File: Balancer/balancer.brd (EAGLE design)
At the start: 170 x 230 mm, 285 parts, among them Q1 BSS123W, Q10A SIR882DP-T1-GE3, Q10B SIS468DN-T1-GE3, Q11A SIR882DP-T1-GE3, Q11B SIS468DN-T1-GE3, Q12A SIR882DP-T1-GE3, Q12B SIS468DN-T1-GE3, Q2 BSS123W, Q3A SIR882DP-T1-GE3, Q3B SIS468DN-T1-GE3, Q4 MMBT3906LT1G, Q4A SIR882DP-T1-GE3, Q4B SIS468DN-T1-GE3, Q5 FDN5618P, Q5A SIR882DP-T1-GE3, Q5B SIS468DN-T1-GE3, Q6 CMPT3904E_TR_PBFREE, Q6A SIR882DP-T1-GE3, Q6B SIS468DN-T1-GE3, Q9A SIR882DP-T1-GE3, Q9B SIS468DN-T1-GE3, T10 750312504, T11 750312504, T12 750312504, T3 750312504, T4 750312504, T5 750312504, T6 750312504, T9 750312504, U1 LTC3300ILXE-1PBF, U2 LTC3300ILXE-1PBF

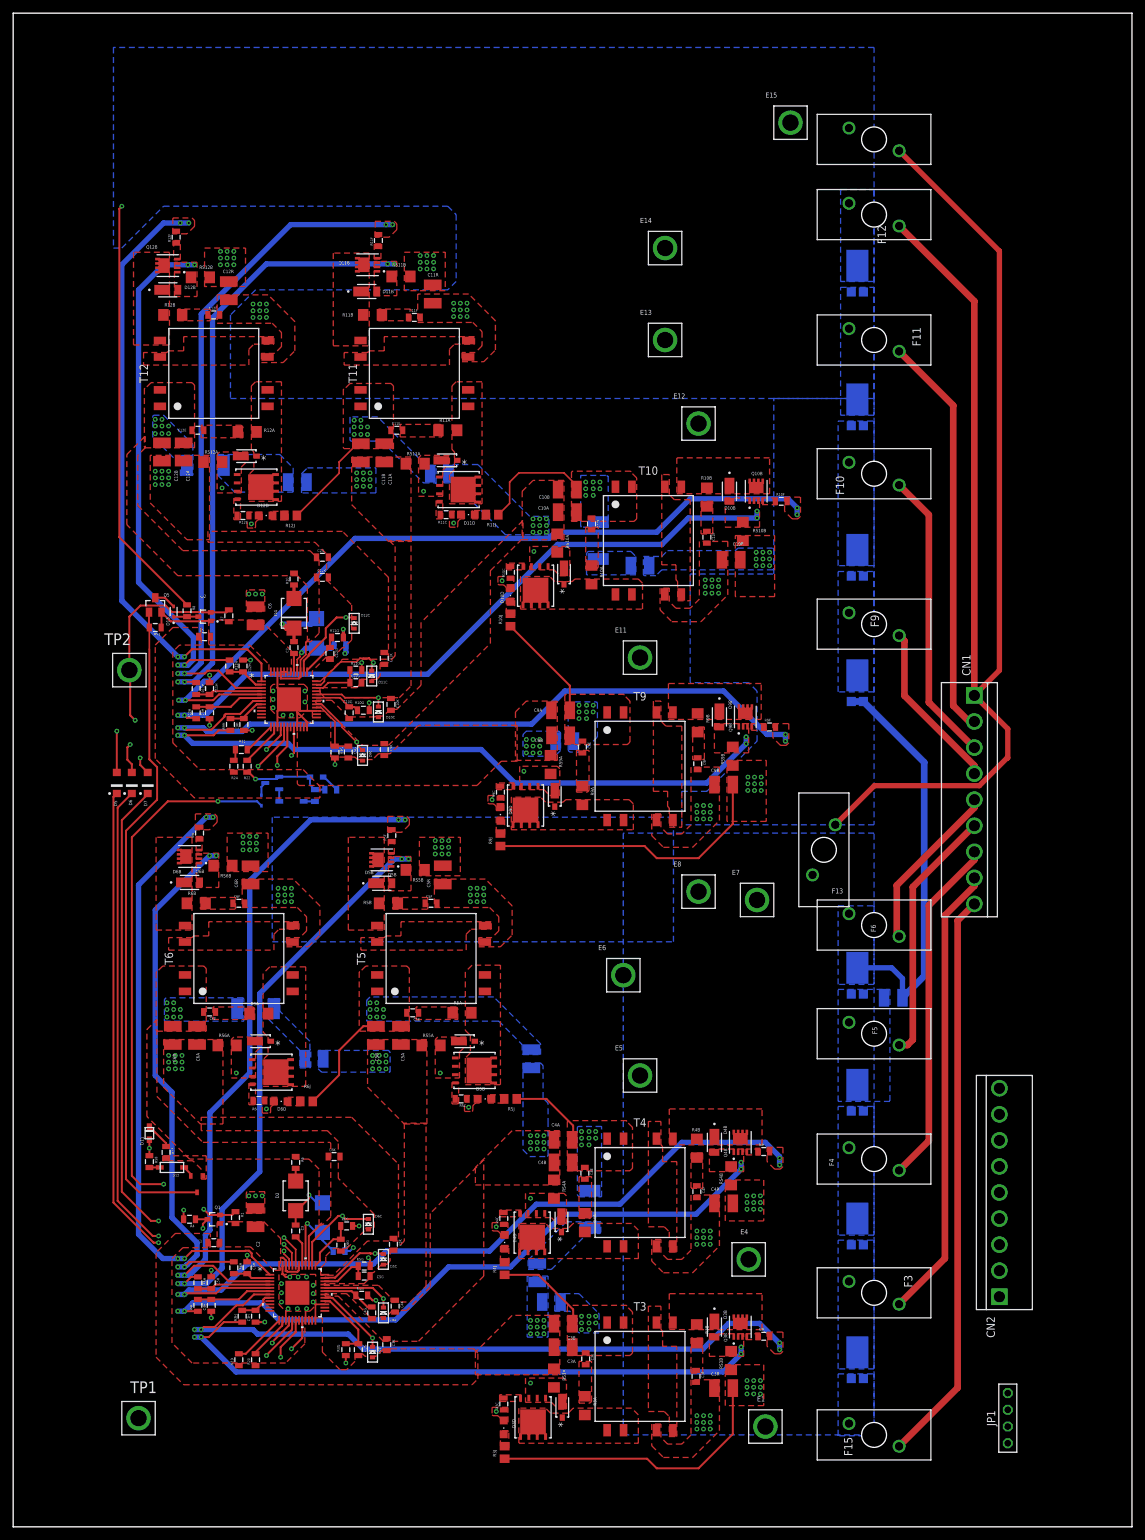
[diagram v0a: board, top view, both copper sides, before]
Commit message: done final check, generated Gerber file
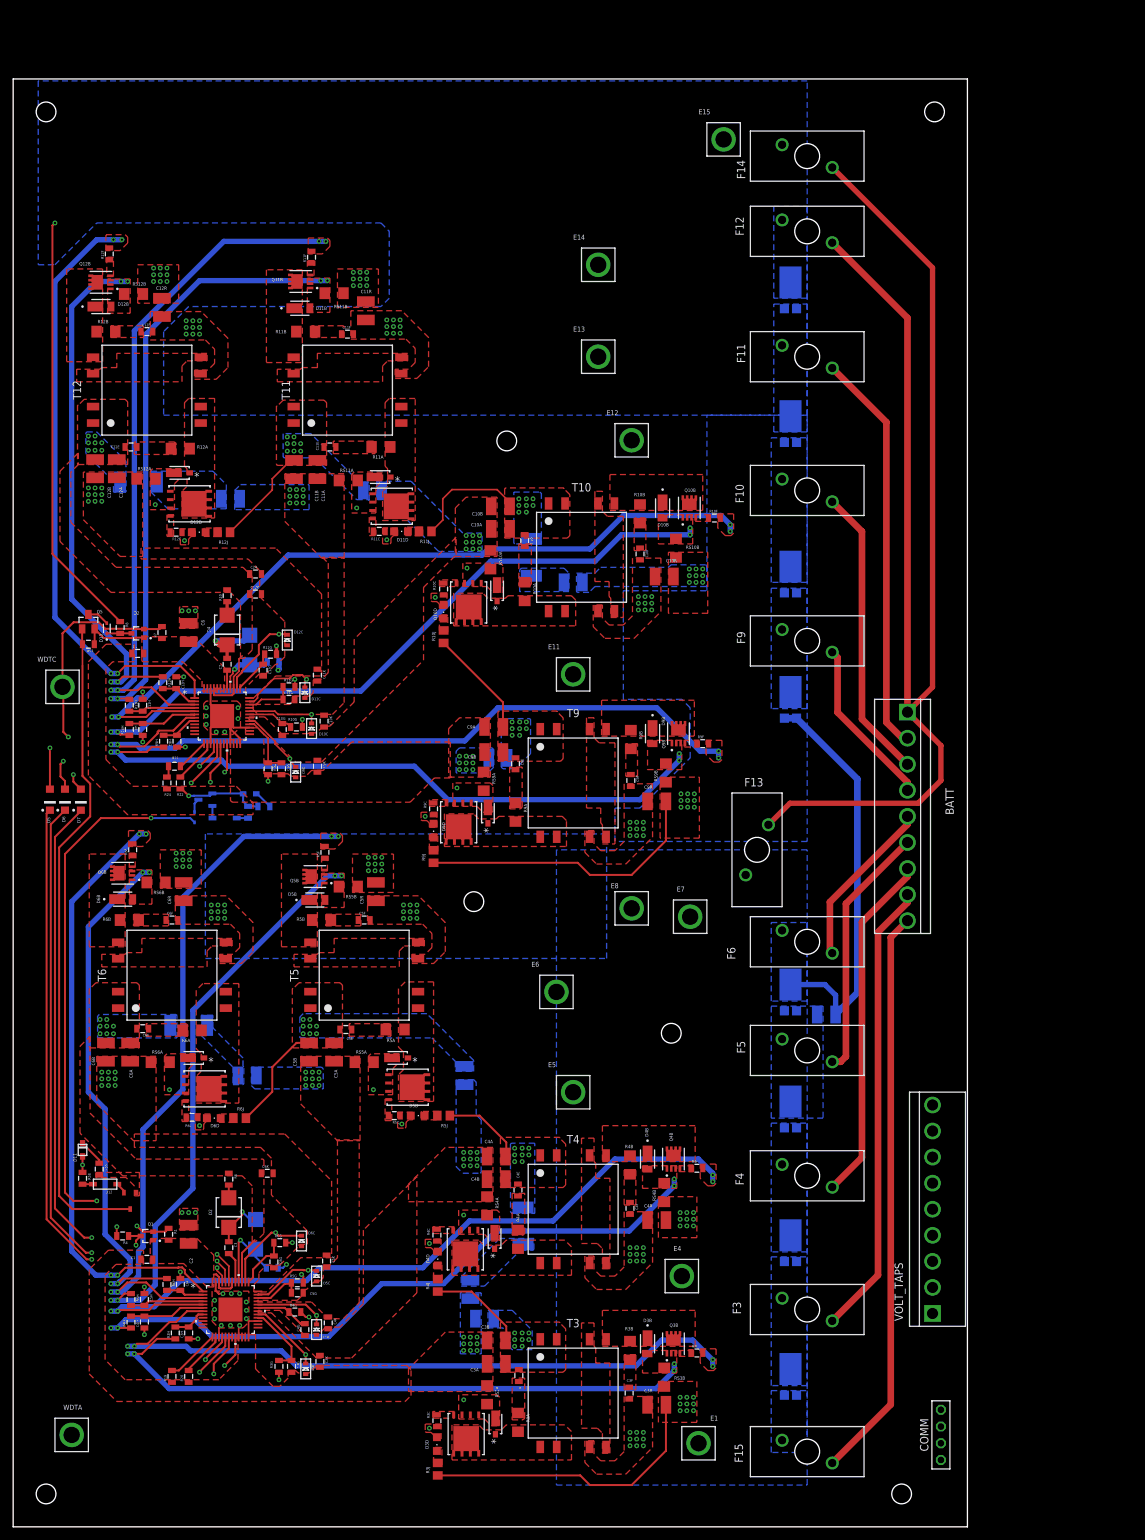
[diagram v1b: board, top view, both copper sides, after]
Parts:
- removed CN1, CN2: (no value), jst-vh:B9P-VH
- removed JP1: PINHD-1X4, Connector:1X04
- removed TP1, TP2: 2501-2-00-80-00-00-07-0, Turret:MILMAX_2501-2-00-80-00-00-07-0
- added BATT, VOLT_TAPS: (no value), jst-vh:B9P-VH
- added COMM: PINHD-1X4, Connector:1X04
- added WDTA, WDTC: 2501-2-00-80-00-00-07-0, Turret:MILMAX_2501-2-00-80-00-00-07-0
- moved D11E 10.5 mm to (118.1, 167.6)
- moved Q10B 10.5 mm to (102.7, 154.8)
- moved R16 10.5 mm to (78.7, 147.3)
- moved RS10A 10.5 mm to (72.5, 146.9)
- moved C3E 10.5 mm to (76.8, 23.0)
- moved D5E 10.5 mm to (118.1, 63.5)
- moved D9A 10.5 mm to (72.1, 108.5)
- moved D9E 10.5 mm to (118.1, 125.7)
- moved R4F 10.5 mm to (103.9, 54.5)
- moved R9B 10.5 mm to (93.9, 119.6)
- moved C11 10.5 mm to (69.5, 36.1)
- moved C9F 10.5 mm to (93.9, 113.4)
- moved D10E 10.5 mm to (118.1, 144.8)
- moved D12E 10.5 mm to (118.1, 188.0)
- moved D3D 10.5 mm to (64.4, 12.6)
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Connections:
- net BAT+: now also BATT.1; no longer CN1.1
- net C10: now also VOLT_TAPS.7; no longer CN2.7
- net C11: now also VOLT_TAPS.8; no longer CN2.8
- net C12: now also VOLT_TAPS.9; no longer CN2.9
- net C3: now also VOLT_TAPS.2; no longer CN2.2
- net C4: now also VOLT_TAPS.3; no longer CN2.3
- net C5: now also VOLT_TAPS.4; no longer CN2.4
- net C6: now also VOLT_TAPS.5; no longer CN2.5
- net C9: now also VOLT_TAPS.6; no longer CN2.6
- net CSBI: now also COMM.3; no longer JP1.3
- net N$14: now also BATT.2; no longer CN1.2
- net N$18: now also BATT.3; no longer CN1.3
- net N$22: now also BATT.4; no longer CN1.4
- net N$23: now also BATT.5; no longer CN1.5
- net N$25: now also BATT.6; no longer CN1.6
- net N$26: now also BATT.7; no longer CN1.7
- net N$28: now also BATT.8; no longer CN1.8
- net N$30: now also BATT.9; no longer CN1.9
- net SCKI: now also COMM.2; no longer JP1.2
- net SDIO: now also COMM.1; no longer JP1.1
- net V-: now also COMM.4, VOLT_TAPS.1; no longer CN2.1, JP1.4
- net WDTA: now also WDTA.1; no longer TP1.1
- net WDTC: now also WDTC.1; no longer TP2.1
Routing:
- net BAT+: track 208.7 -> 208.2 mm
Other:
- board size 170 x 230 mm -> 145 x 220 mm
